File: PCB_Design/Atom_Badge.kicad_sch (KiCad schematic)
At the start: 51 parts

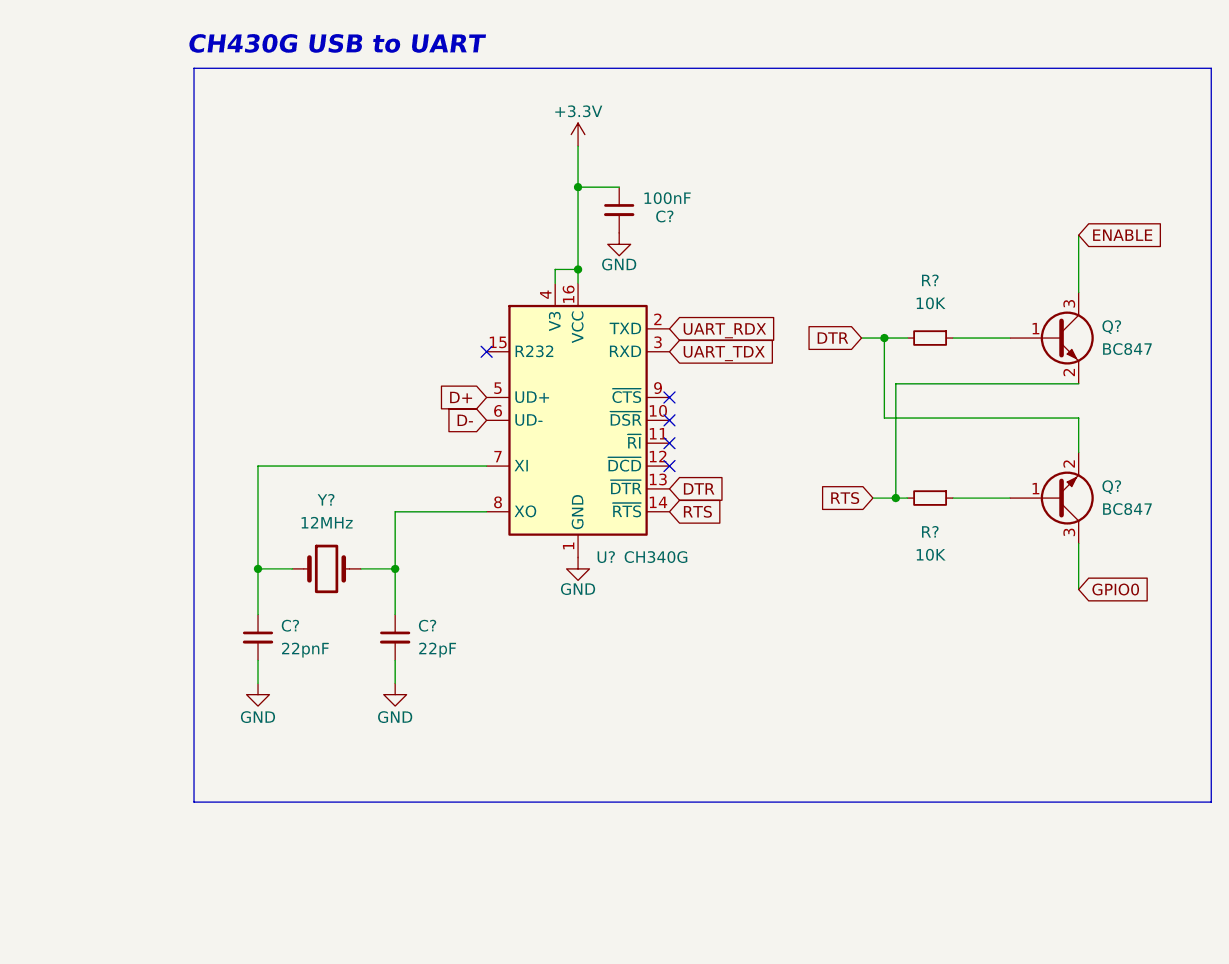
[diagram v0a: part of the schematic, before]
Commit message: new transistor
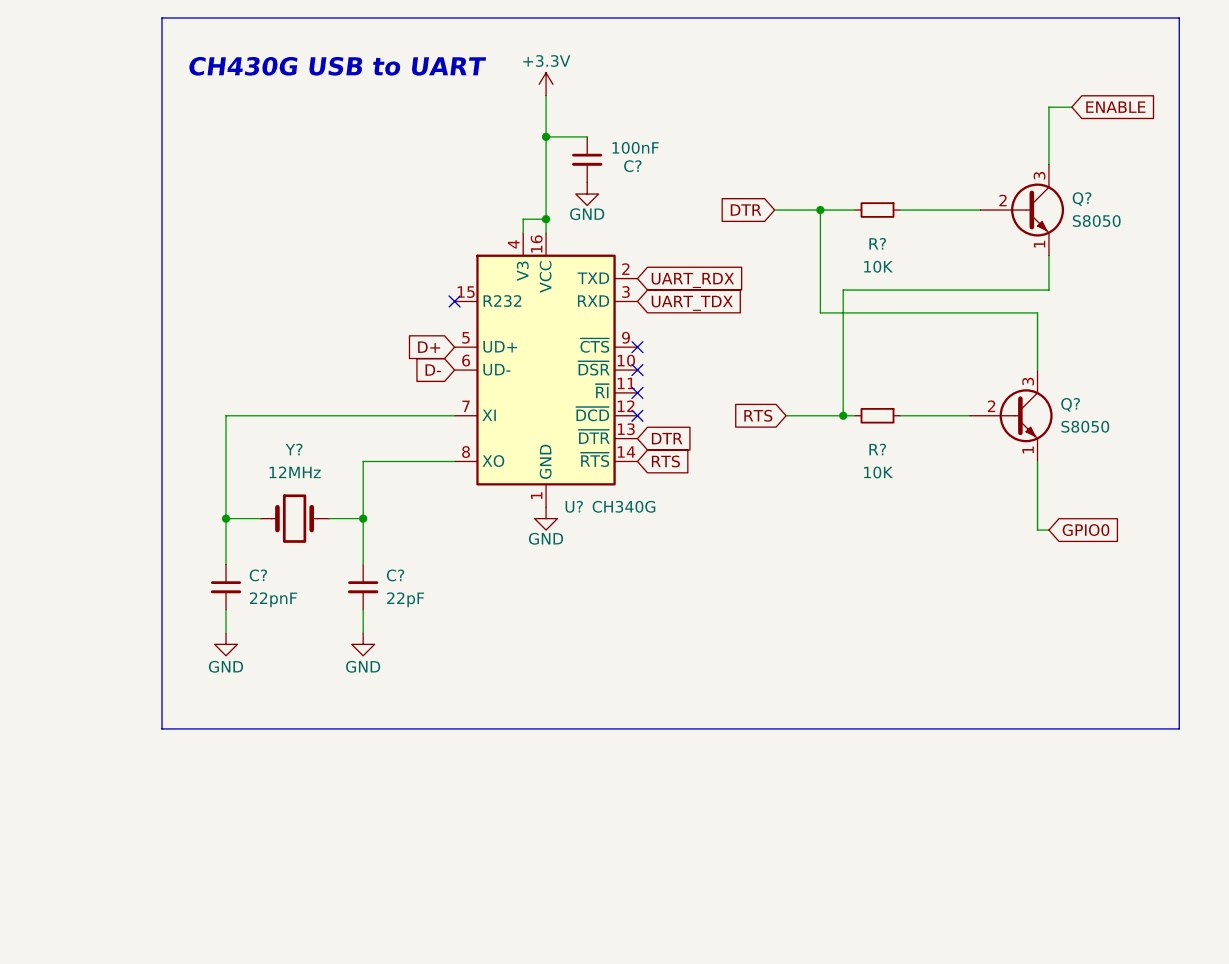
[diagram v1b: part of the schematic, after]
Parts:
- removed Q? (x2): BC847, Package_TO_SOT_SMD:SOT-23, symbol Transistor_BJT:BC847
- removed R? (x2): 10K, symbol Device:R_Small
- added Q? (x2): S8050, Package_TO_SOT_THT:TO-92_Inline, symbol Transistor_BJT:S8050
- added R? (x2): 10K, symbol Device:R_Small
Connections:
- net DTR: now also Q?.3 (C), R?.2
- net ENABLE: now also Q?.3 (C)
- net GPIO0: now also Q?.1 (E)
- net RTS: now also Q?.1 (E), R?.2
- new net: Q?.2 (B), R?.1 (x2)
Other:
- moved on the sheet: C?, U?, Y?
